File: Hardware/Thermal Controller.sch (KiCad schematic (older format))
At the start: 8 parts, among them M1 Fan, U1 TB6643KQ, U2 RC1602A, U3 TB6643KQ

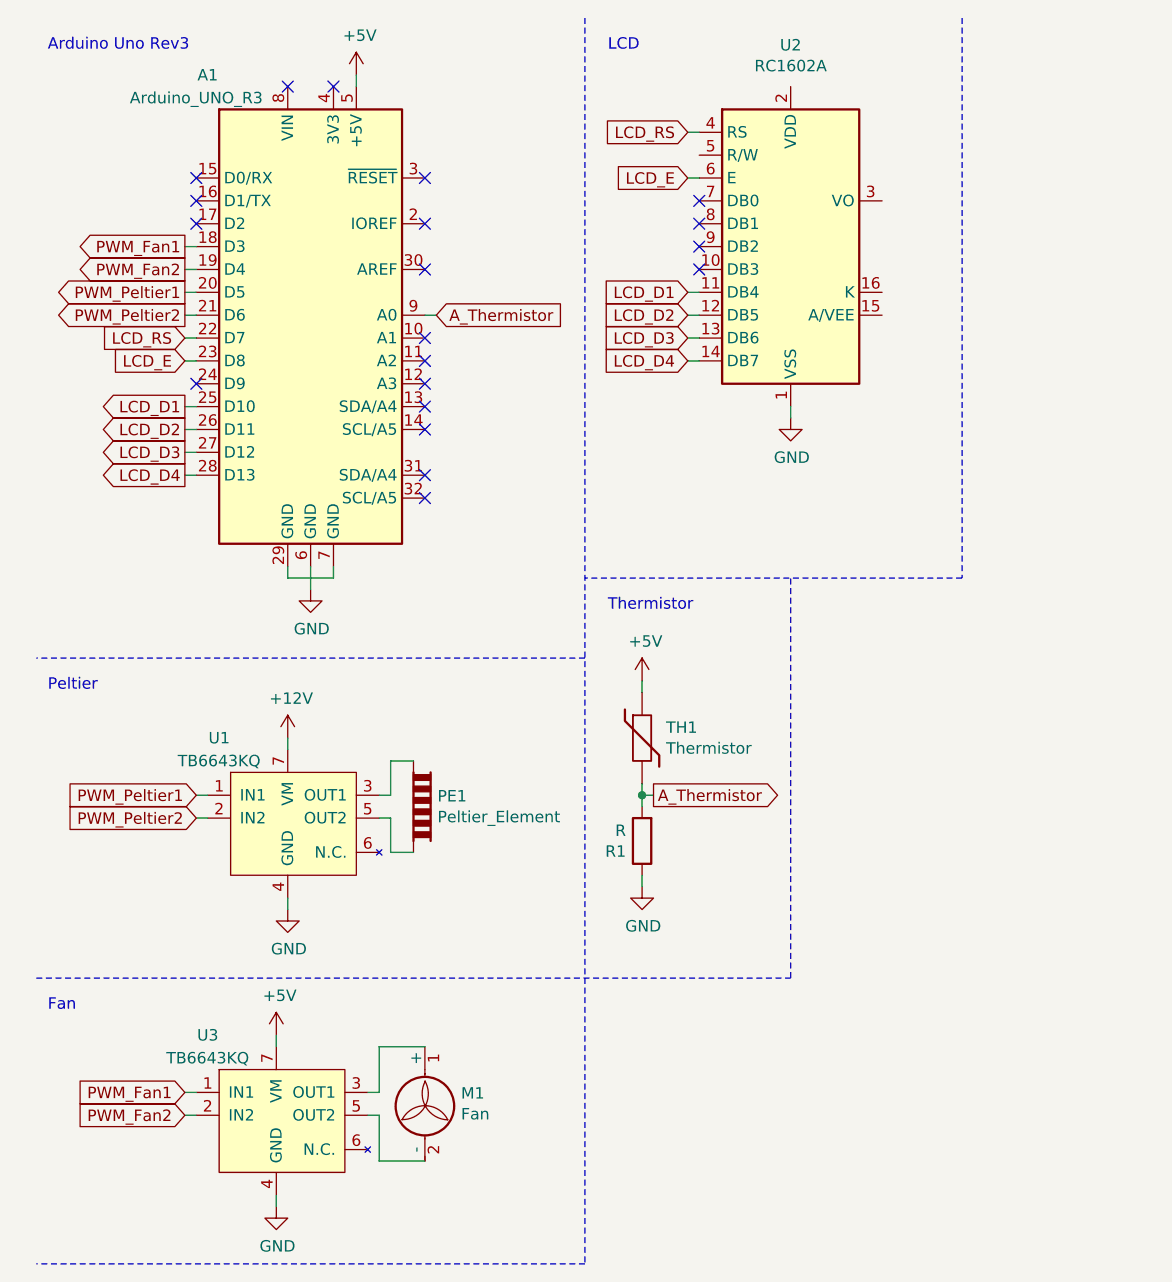
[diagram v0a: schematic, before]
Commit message: Add files via upload
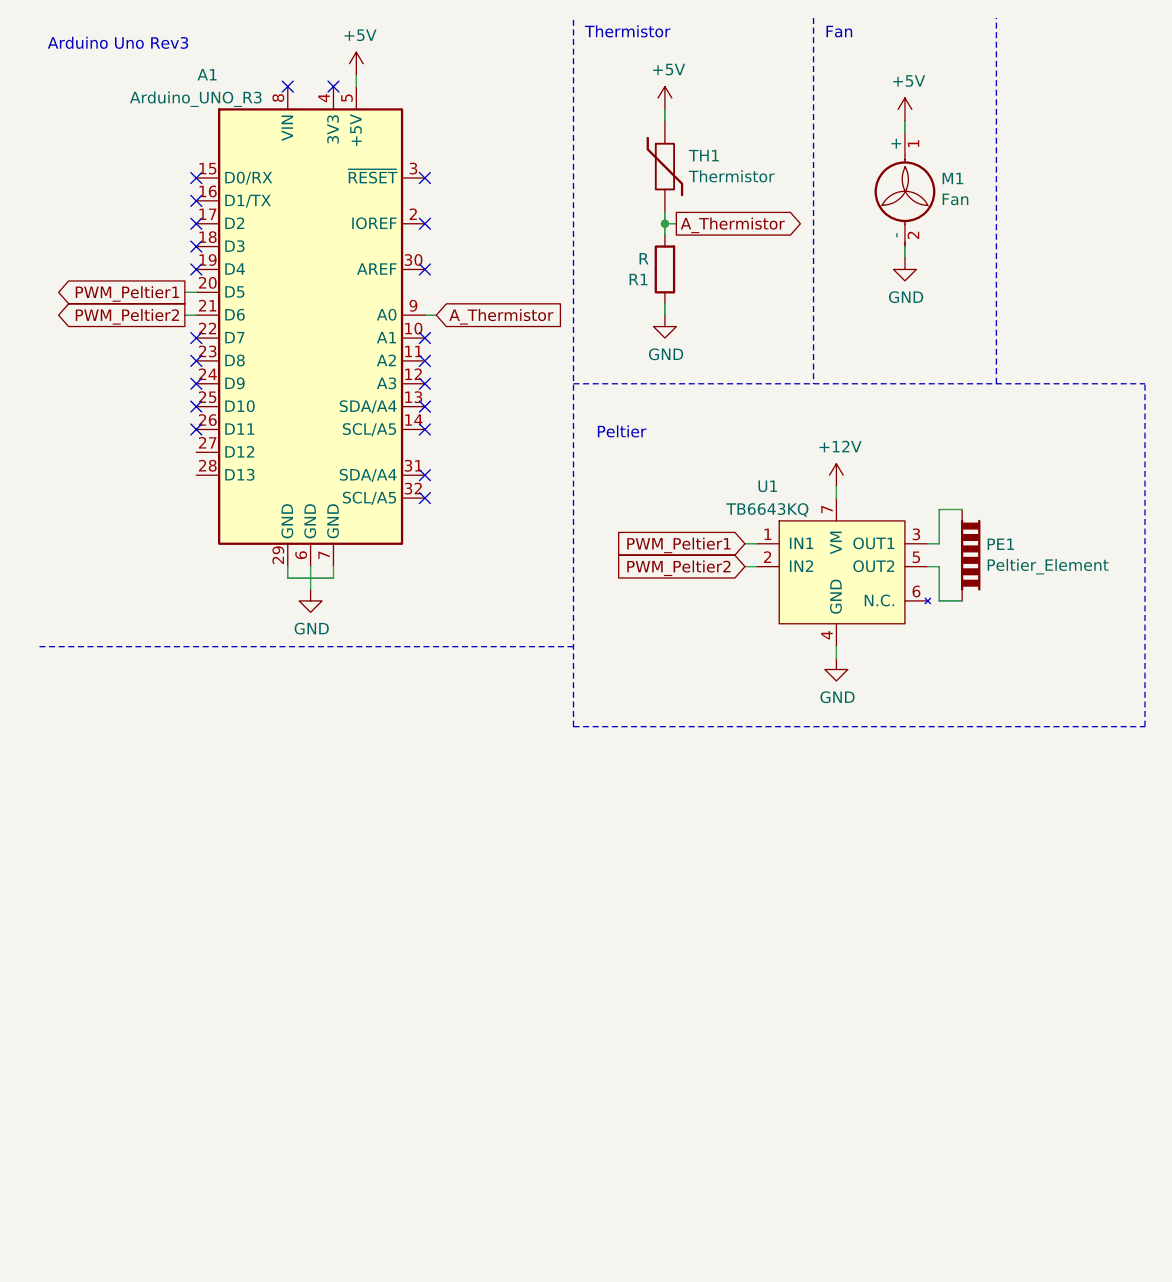
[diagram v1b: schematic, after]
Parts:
- removed U2: RC1602A, Display:RC1602A, symbol Display_Character:RC1602A
- removed U3: TB6643KQ, Connector_PinSocket_2.54mm:PinSocket_1x07_P2.54mm_Vertical, symbol Thermal-Controller-rescue:TB6643KQ-Themal_Controller
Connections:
- net +5V: now also M1.1 (+)
- net GND: now also M1.2 (-)
- net LCD_D1: no longer names the net of A1.25 (D10)
- net LCD_D2: no longer names the net of A1.26 (D11)
- net LCD_D3: no longer names the net of A1.27 (D12)
- net LCD_D4: no longer names the net of A1.28 (D13)
- net LCD_E: no longer names the net of A1.23 (D8)
- net LCD_RS: no longer names the net of A1.22 (D7)
- net PWM_Fan1: no longer names the net of A1.18 (D3)
- net PWM_Fan2: no longer names the net of A1.19 (D4)
- no-connect marks 20 -> 22
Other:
- note removed: "LCD\n"
- moved on the sheet: M1, PE1, R1, TH1, U1
